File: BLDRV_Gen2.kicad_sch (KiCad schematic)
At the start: 46 parts, among them J1 Conn_01x03_Pin, J3 Pin, J4 Pin, P1 USB_C_Plug_USB2.0, SW1 SW_Push, SW2 SW_SPDT, U1 STM32F303K8Tx, U2 DRV8316CTRGFR, U4 NJM2845DL1, U7 AS5048A, U8 CH340E

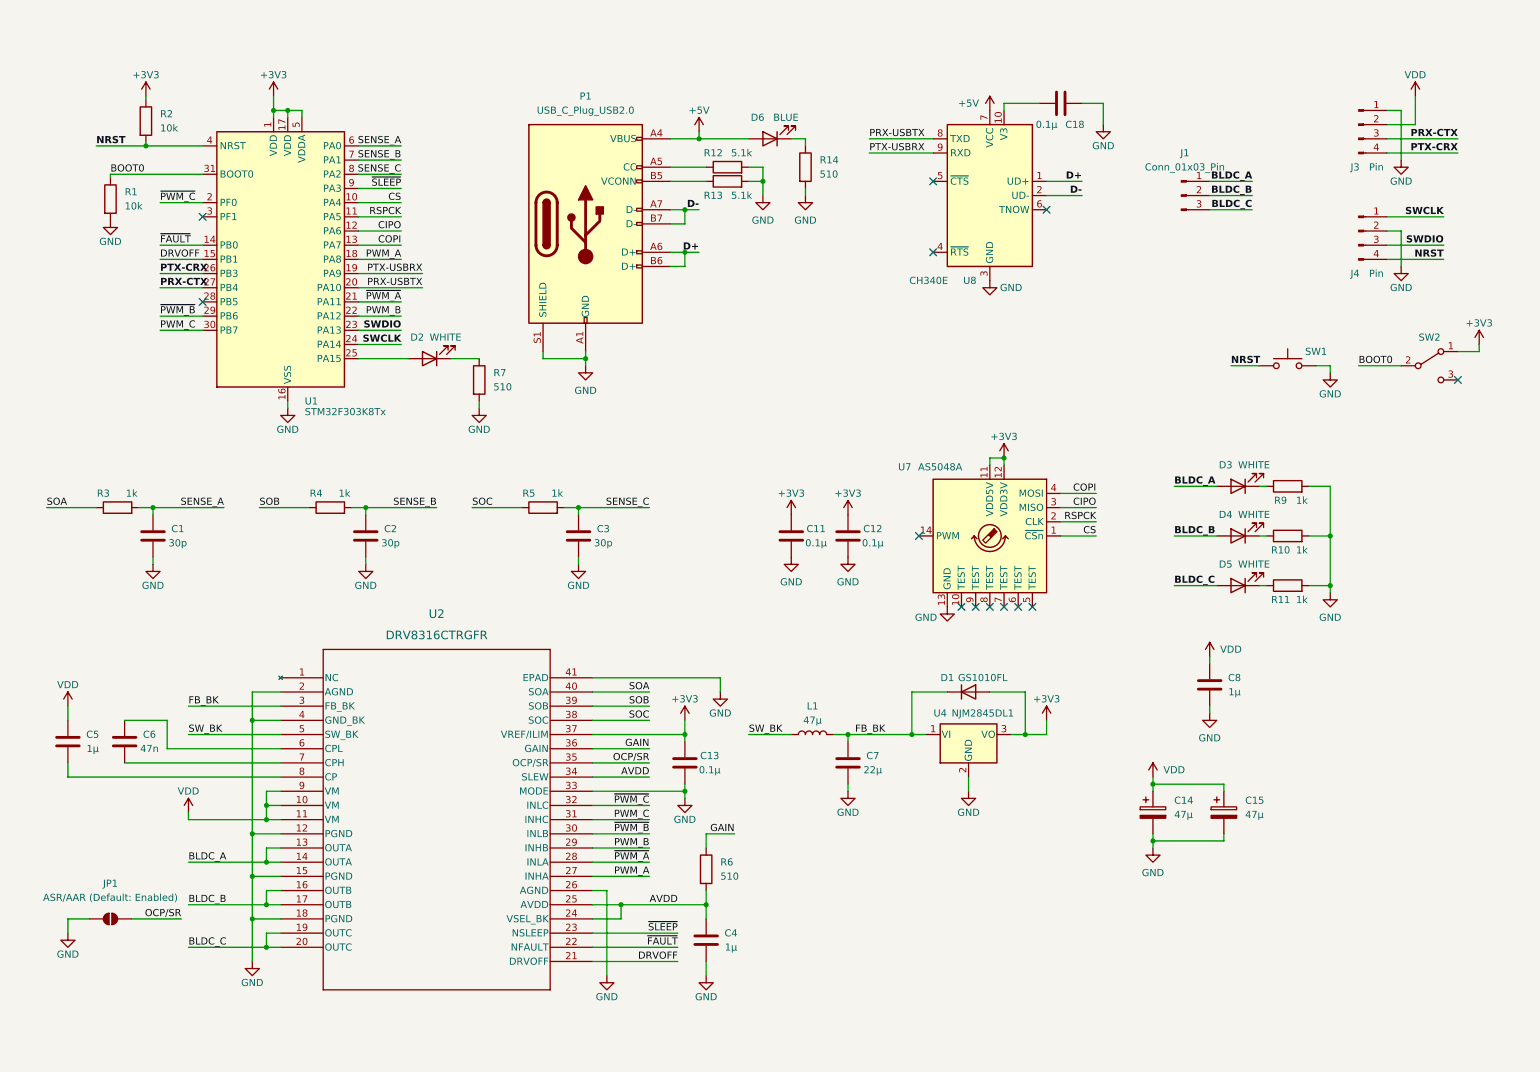
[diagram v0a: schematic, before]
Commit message: ♻️ 回路図
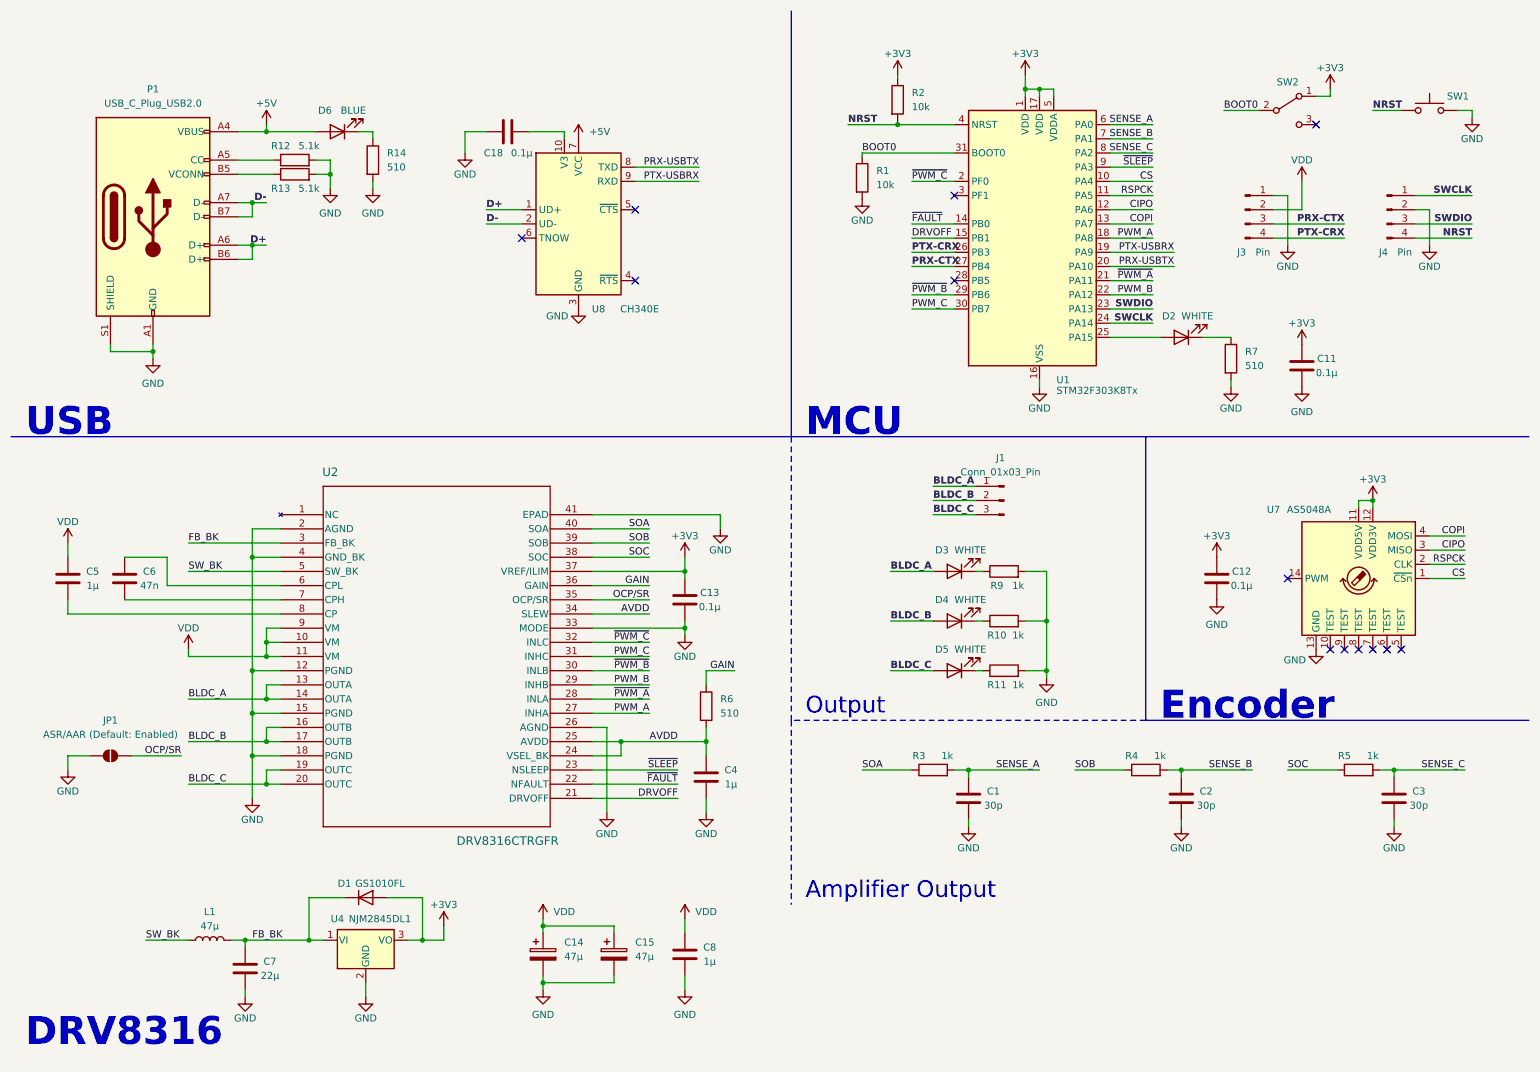
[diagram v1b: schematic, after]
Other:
- note added: "Amplifier Output"
- note added: "DRV8316"
- note added: "Encoder"
- note added: "MCU"
- note added: "Output"
- note added: "USB"
- moved on the sheet: C1, C11, C12, C13, C14, C15, C18, C2, C3, C4, C5, C6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
